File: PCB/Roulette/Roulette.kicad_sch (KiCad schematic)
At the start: 277 parts, among them J1 USB-PROG, J2 Shelly, J3 Conn_01x03, J3 JST-PH-SM3-TBT, J4 Conn_01x02, J6 C3001289, Q1 C179347, Q4 CJ2301, SW1 SW_Push, U2 ESP32-S3-MINI-1, U2 ME6211C33M5G-N, U5 TP4054

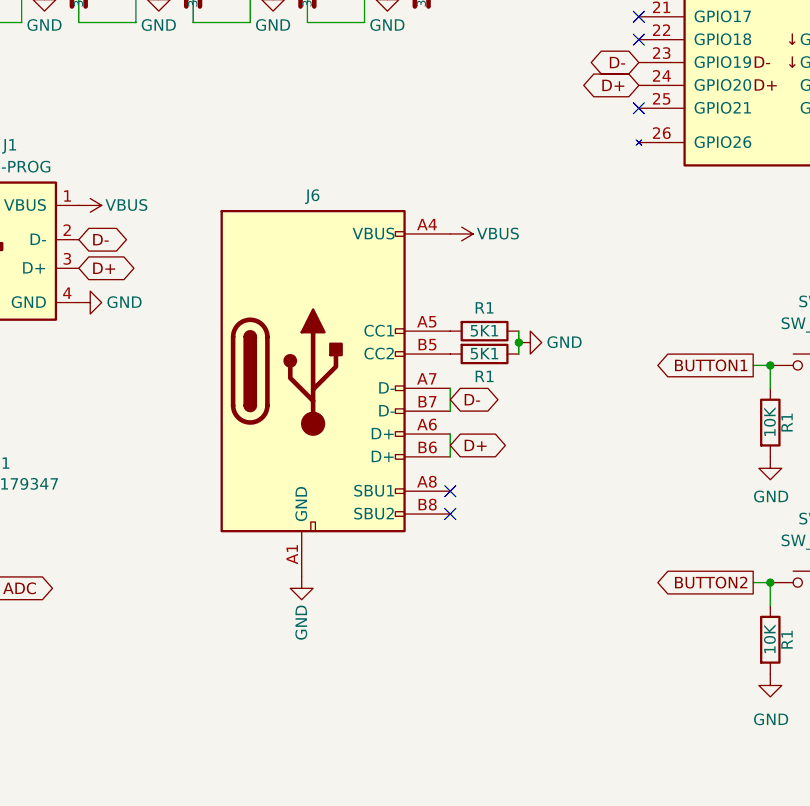
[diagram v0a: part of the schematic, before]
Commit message: Part IDs
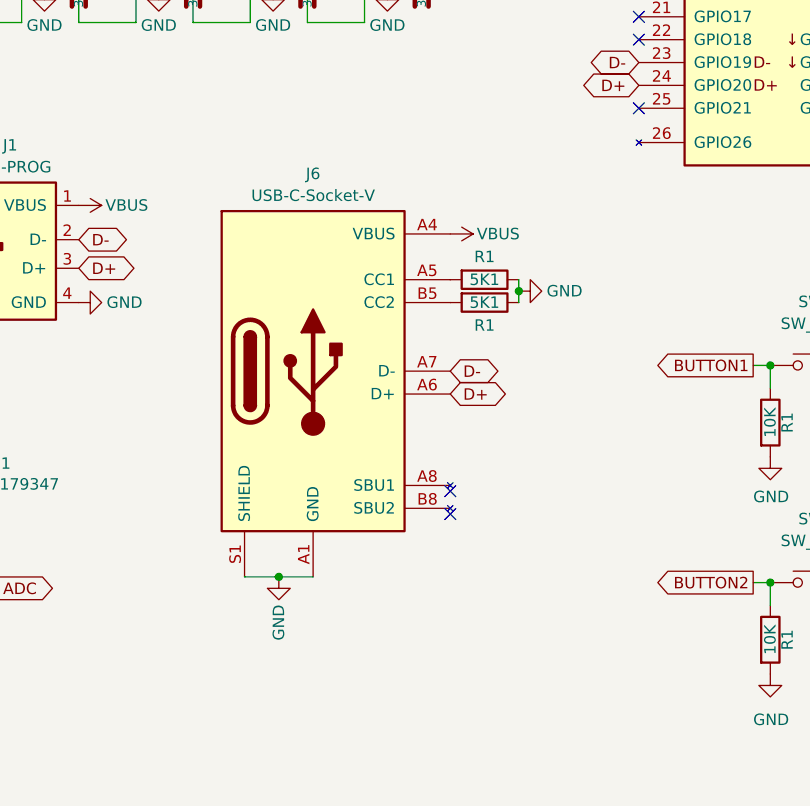
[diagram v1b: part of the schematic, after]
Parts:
- removed J6: C3001289, RevK:USB_C_G_Switch-7082A, symbol RevK:USB_C_Receptacle_G_Switch_7082C
- added J6: USB-C-Socket-V, RevK:USB_C_G_Switch-7082A, symbol RevK:USB-C-Socket-V
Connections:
- net D+: now also J6.A6 (D+), J6.B6 (D+)
- net D-: now also J6.A7 (D-), J6.B7 (D-)
- net GND: now also J6.A1 (GND), J6.A12 (GND), J6.B1 (GND), J6.B12 (GND), J6.S1 (SHIELD)
- net VBUS: now also J6.A4 (VBUS), J6.A9 (VBUS), J6.B4 (VBUS), J6.B9 (VBUS)
- net at R1.2: now also J6.B5 (CC2)
- net at R1.2: now also J6.A5 (CC1)
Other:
- moved on the sheet: R1
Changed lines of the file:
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@@
   (junction (at 31.75 31.115) (diameter 0) (color 0 0 0 0)
   )
+  (junction (at 196.85 148.59) (diameter 0) (color 0 0 0 0)
+  )
   (junction (at 178.435 76.835) (diameter 0) (color 0 0 0 0)
   )
@@
   (junction (at 178.435 24.765) (diameter 0) (color 0 0 0 0)
   )
-  (junction (at 223.52 122.555) (diameter 0) (color 0 0 0 0)
+  (junction (at 223.52 116.84) (diameter 0) (color 0 0 0 0)
   )
   (junction (at -3.175 88.265) (diameter 0) (color 0 0 0 0)
@@
     (stroke (width 0) (type default))
   )
-  (wire (pts (xy 215.9 127.635) (xy 215.9 130.175))
-    (stroke (width 0) (type default))
-  )
   (wire (pts (xy 16.51 28.575) (xy 16.51 33.655))
     (stroke (width 0) (type default))
@@
     (stroke (width 0) (type default))
   )
+  (wire (pts (xy 193.04 148.59) (xy 196.85 148.59))
+    (stroke (width 0) (type default))
+  )
   (wire (pts (xy 24.13 75.565) (xy 24.13 81.915))
     (stroke (width 0) (type default))
@@
     (stroke (width 0) (type default))
   )
-  (wire (pts (xy 215.9 132.715) (xy 215.9 135.255))
-    (stroke (width 0) (type default))
-  )
   (wire (pts (xy 12.7 31.115) (xy 12.7 37.465))
     (stroke (width 0) (type default))
@@
     (stroke (width 0) (type default))
   )
-  (wire (pts (xy 223.52 122.555) (xy 223.52 123.825))
+  (wire (pts (xy 223.52 116.84) (xy 223.52 118.11))
     (stroke (width 0) (type default))
   )
@@
     (stroke (width 0) (type default))
   )
-  (wire (pts (xy 223.52 121.285) (xy 223.52 122.555))
+  (wire (pts (xy 223.52 115.57) (xy 223.52 116.84))
     (stroke (width 0) (type default))
   )
@@
     (stroke (width 0) (type default))
   )
+  (wire (pts (xy 196.85 148.59) (xy 200.66 148.59))
+    (stroke (width 0) (type default))
+  )
   (wire (pts (xy 94.615 46.355) (xy 94.615 53.975))
     (stroke (width 0) (type default))
@@
     )
   )
-  (global_label "D+" (shape bidirectional) (at 215.9 133.985 0) (fields_autoplaced)
+  (global_label "D+" (shape bidirectional) (at 215.9 128.27 0) (fields_autoplaced)
     (effects (font (size 1.27 1.27)) (justify left))
-    (property "Intersheetrefs" "${INTERSHEET_REFS}" (at 221.9465 133.985 0)
+    (property "Intersheetrefs" "${INTERSHEET_REFS}" (at 221.9465 128.27 0)
       (effects (font (size 1.27 1.27)) (justify left) hide)
     )
@@
     )
   )
-  (global_label "D-" (shape bidirectional) (at 215.9 128.905 0) (fields_autoplaced)
+  (global_label "D-" (shape bidirectional) (at 215.9 125.73 0) (fields_autoplaced)
     (effects (font (size 1.27 1.27)) (justify left))
-    (property "Intersheetrefs" "${INTERSHEET_REFS}" (at 221.9465 128.905 0)
+    (property "Intersheetrefs" "${INTERSHEET_REFS}" (at 221.9465 125.73 0)
       (effects (font (size 1.27 1.27)) (justify left) hide)
     )
@@
     )
   )
-  (symbol (lib_id "power:GND") (at 223.52 122.555 90) (unit 1)
+  (symbol (lib_id "power:GND") (at 223.52 116.84 90) (unit 1)
     (in_bom yes) (on_board yes) (dnp no)
-    (property "Reference" "#PWR045" (at 229.87 122.555 0)
+    (property "Reference" "#PWR045" (at 229.87 116.84 0)
       (effects (font (size 1.27 1.27)) hide)
     )
-    (property "Value" "GND" (at 228.6 122.555 90)
+    (property "Value" "GND" (at 228.6 116.84 90)
       (effects (font (size 1.27 1.27)))
     )
-    (property "Footprint" "" (at 223.52 122.555 0)
+    (property "Footprint" "" (at 223.52 116.84 0)
       (effects (font (size 1.27 1.27)) hide)
     )
-    (property "Datasheet" "" (at 223.52 122.555 0)
+    (property "Datasheet" "" (at 223.52 116.84 0)
       (effects (font (size 1.27 1.27)) hide)
     )
@@
     )
   )
-  (symbol (lib_id "Device:R") (at 219.71 123.825 270) (unit 1)
+  (symbol (lib_id "Device:R") (at 219.71 118.11 270) (unit 1)
     (in_bom yes) (on_board yes) (dnp no)
-    (property "Reference" "R1" (at 219.71 126.365 90)
+    (property "Reference" "R1" (at 219.71 120.65 90)
       (effects (font (size 1.27 1.27)))
     )
-    (property "Value" "5K1" (at 219.71 123.825 90)
+    (property "Value" "5K1" (at 219.71 118.11 90)
       (effects (font (size 1.27 1.27)))
     )
-    (property "Footprint" "RevK:R_0402" (at 219.71 122.047 90)
+    (property "Footprint" "RevK:R_0402" (at 219.71 116.332 90)
       (effects (font (size 1.27 1.27)) hide)
     )
-    (property "Datasheet" "~" (at 219.71 123.825 0)
+    (property "Datasheet" "~" (at 219.71 118.11 0)
       (effects (font (size 1.27 1.27)) hide)
     )
@@
     )
   )
+  (symbol (lib_id "RevK:USB-C-Socket-V") (at 200.66 125.73 0) (unit 1)
+    (in_bom yes) (on_board yes) (dnp no) (fields_autoplaced)
+    (property "Reference" "J6" (at 200.66 103.8057 0)
+      (effects (font (size 1.27 1.27)))
+    )
+    (property "Value" "USB-C-Socket-V" (at 200.66 106.2299 0)
+      (effects (font (size 1.27 1.27)))
+    )
+    (property "Footprint" "RevK:USB_C_G_Switch-7082A" (at 200.66 105.41 0)
+      (effects (font (size 1.27 1.27)) hide)
+    )
+    (property "Datasheet" "" (at 200.66 102.87 0)
+      (effects (font (size 1.27 1.27)) hide)
+    )
+    (property "LCSC Part #" "C709357" (at 200.66 125.73 0)
+      (effects (font (size 1.27 1.27)) hide)
+    )
+    (pin "A1")
+    (pin "A12")
+    (pin "A4")
+    (pin "A5")
+    (pin "A6")
+    (pin "A7")
+    (pin "A8")
+    (pin "A9")
+    (pin "B1")
+    (pin "B12")
+    (pin "B4")
+    (pin "B5")
+    (pin "B6")
+    (pin "B7")
+    (pin "B8")
+    (pin "B9")
+    (pin "S1")
+    (instances
+      (project "Roulette"
+        (path "/46c350bb-7de4-4e81-aafd-4af55e37aab0"
+          (reference "J6") (unit 1)
+        )
+      )
+    )
+  )
   (symbol (lib_id "Device:R") (at 251.46 131.445 0) (unit 1)
     (in_bom yes) (on_board yes) (dnp no)
@@
     )
   )
-  (symbol (lib_id "RevK:USB_C_Receptacle_G_Switch_7082C") (at 200.66 125.73 0) (unit 1)
-    (in_bom yes) (on_board yes) (dnp no) (fields_autoplaced)
-    (property "Reference" "J6" (at 200.66 106.2299 0)
-      (effects (font (size 1.27 1.27)))
-    )
-    (property "Value" "C3001289" (at 200.66 106.2299 0)
-      (effects (font (size 1.27 1.27)) hide)
-    )
-    (property "Footprint" "RevK:USB_C_G_Switch-7082A" (at 204.47 125.73 0)
-      (effects (font (size 1.27 1.27)) hide)
-    )
-    (property "Datasheet" "https://www.usb.org/sites/default/files/documents/usb_type-c.zip" (at 204.47 125.73 0)
-      (effects (font (size 1.27 1.27)) hide)
-    )
-    (property "LCSC Part #" "C3001289" (at 200.66 125.73 0)
-      (effects (font (size 1.27 1.27)) hide)
-    )
-    (pin "A1")
-    (pin "A12")
-    (pin "A4")
-    (pin "A5")
-    (pin "A6")
-    (pin "A7")
-    (pin "A8")
-    (pin "A9")
-    (pin "B1")
-    (pin "B12")
-    (pin "B4")
-    (pin "B5")
-    (pin "B6")
-    (pin "B7")
-    (pin "B8")
-    (pin "B9")
-    (instances
-      (project "Roulette"
-        (path "/46c350bb-7de4-4e81-aafd-4af55e37aab0"
-          (reference "J6") (unit 1)
-        )
-      )
-    )
-  )
   (symbol (lib_id "Device:C") (at 62.23 81.915 270) (mirror x) (unit 1)
     (in_bom yes) (on_board yes) (dnp no)
@@
     )
   )
-  (symbol (lib_id "power:GND") (at 199.39 148.59 0) (unit 1)
+  (symbol (lib_id "power:GND") (at 196.85 148.59 0) (unit 1)
     (in_bom yes) (on_board yes) (dnp no)
-    (property "Reference" "#PWR021" (at 199.39 154.94 0)
+    (property "Reference" "#PWR021" (at 196.85 154.94 0)
       (effects (font (size 1.27 1.27)) hide)
     )
-    (property "Value" "GND" (at 199.39 153.67 90)
+    (property "Value" "GND" (at 196.85 153.67 90)
       (effects (font (size 1.27 1.27)))
     )
-    (property "Footprint" "" (at 199.39 148.59 0)
+    (property "Footprint" "" (at 196.85 148.59 0)
       (effects (font (size 1.27 1.27)) hide)
     )
-    (property "Datasheet" "" (at 199.39 148.59 0)
+    (property "Datasheet" "" (at 196.85 148.59 0)
       (effects (font (size 1.27 1.27)) hide)
     )
@@
     )
   )
-  (symbol (lib_id "Device:R") (at 219.71 121.285 270) (unit 1)
+  (symbol (lib_id "Device:R") (at 219.71 115.57 270) (unit 1)
     (in_bom yes) (on_board yes) (dnp no)
-    (property "Reference" "R1" (at 219.71 118.745 90)
+    (property "Reference" "R1" (at 219.71 113.03 90)
       (effects (font (size 1.27 1.27)))
     )
-    (property "Value" "5K1" (at 219.71 121.285 90)
+    (property "Value" "5K1" (at 219.71 115.57 90)
       (effects (font (size 1.27 1.27)))
     )
-    (property "Footprint" "RevK:R_0402" (at 219.71 119.507 90)
+    (property "Footprint" "RevK:R_0402" (at 219.71 113.792 90)
       (effects (font (size 1.27 1.27)) hide)
     )
-    (property "Datasheet" "~" (at 219.71 121.285 0)
+    (property "Datasheet" "~" (at 219.71 115.57 0)
       (effects (font (size 1.27 1.27)) hide)
     )
